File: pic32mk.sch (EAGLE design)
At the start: 31 parts, among them IC1 PIC32MK1024MCF100-I_PT, IC2 ADM3095EBRZ, IC3 PIC32MK1024MCF100-I_PT, IC4 MAX203ECWP

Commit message: up
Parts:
- added SV1: ICSP1, con-lstb:MA06-1
- added SV2: ICSP2, con-lstb:MA06-1
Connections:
- new net N$11: IC3.PGED1/OA1IN-/AN5/CTCMP/C1IN1-/RTCC/RPB3/RB3, SV1.4
- new net N$12: IC3.PGEC1/OA1IN+/AN4/C1IN1+/C1IN3-/C2IN3-/RPB2/RB2, SV1.5
- new net N$13: IC1.PGED1/OA1IN-/AN5/CTCMP/C1IN1-/RTCC/RPB3/RB3, SV2.4
- new net N$14: IC1.PGEC1/OA1IN+/AN4/C1IN1+/C1IN3-/C2IN3-/RPB2/RB2, SV2.5
- net +3V3: now also SV1.3, SV2.3
- net N$2: now also SV2.1
- net N$5: now also SV1.1
- net VSS: now also SV1.2, SV2.2
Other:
- moved on the sheet: U$1
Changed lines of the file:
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@@
 <class number="0" name="default" width="0" drill="0">
 </class>
-<class number="1" name="icurrent" width="0.0127" drill="0">
+<class number="1" name="icurrent" width="0.2159" drill="0">
 </class>
 </classes>
@@
 <part name="VSS25" library="supply1" library_urn="urn:adsk.eagle:library:371" deviceset="VSS" device=""/>
 <part name="VSS26" library="supply1" library_urn="urn:adsk.eagle:library:371" deviceset="VSS" device=""/>
+<part name="SV1" library="con-lstb" library_urn="urn:adsk.eagle:library:162" deviceset="MA06-1" device="" package3d_urn="urn:adsk.eagle:package:8340/1" value="ICSP1"/>
+<part name="VSS27" library="supply1" library_urn="urn:adsk.eagle:library:371" deviceset="VSS" device=""/>
+<part name="+3V2" library="supply1" library_urn="urn:adsk.eagle:library:371" deviceset="+3V3" device=""/>
+<part name="SV2" library="con-lstb" library_urn="urn:adsk.eagle:library:162" deviceset="MA06-1" device="" package3d_urn="urn:adsk.eagle:package:8340/1" value="ICSP2"/>
+<part name="VSS28" library="supply1" library_urn="urn:adsk.eagle:library:371" deviceset="VSS" device=""/>
+<part name="+3V3" library="supply1" library_urn="urn:adsk.eagle:library:371" deviceset="+3V3" device=""/>
 </parts>
 <sheets>
@@
 <attribute name="VALUE" x="208.28" y="-127" size="1.778" layer="96"/>
 </instance>
-<instance part="U$1" gate="G$1" x="-43.18" y="-101.6" smashed="yes">
-<attribute name="VALUE" x="-50.81086875" y="-88.8819" size="2.54361875" layer="96"/>
-<attribute name="NAME" x="-61.009" y="-65.942" size="1.7829" layer="95"/>
+<instance part="U$1" gate="G$1" x="-66.04" y="-99.06" smashed="yes">
+<attribute name="VALUE" x="-73.67086875" y="-86.3419" size="2.54361875" layer="96"/>
+<attribute name="NAME" x="-83.869" y="-63.402" size="1.7829" layer="95"/>
 </instance>
 <instance part="U$2" gate="G$1" x="-124.46" y="416.56" smashed="yes">
@@
 <attribute name="VALUE" x="-121.285" y="342.265" size="1.778" layer="96"/>
 </instance>
-<instance part="SUPPLY2" gate="GND" x="-43.18" y="-139.7" smashed="yes">
-<attribute name="VALUE" x="-45.085" y="-142.875" size="1.778" layer="96"/>
-</instance>
-<instance part="P+4" gate="VCC" x="-43.18" y="-63.5" smashed="yes">
-<attribute name="VALUE" x="-45.72" y="-66.04" size="1.778" layer="96" rot="R90"/>
+<instance part="SUPPLY2" gate="GND" x="-66.04" y="-137.16" smashed="yes">
+<attribute name="VALUE" x="-67.945" y="-140.335" size="1.778" layer="96"/>
+</instance>
+<instance part="P+4" gate="VCC" x="-66.04" y="-58.42" smashed="yes">
+<attribute name="VALUE" x="-68.58" y="-60.96" size="1.778" layer="96" rot="R90"/>
 </instance>
 <instance part="C10" gate="G$1" x="-96.52" y="365.76" smashed="yes">
@@
 <instance part="VSS26" gate="G$1" x="-86.36" y="358.14" smashed="yes">
 <attribute name="VALUE" x="-88.9" y="353.06" size="1.778" layer="96" rot="R90"/>
+</instance>
+<instance part="SV1" gate="1" x="-63.5" y="200.66" smashed="yes">
+<attribute name="VALUE" x="-64.77" y="187.96" size="1.778" layer="96"/>
+<attribute name="NAME" x="-64.77" y="209.042" size="1.778" layer="95"/>
+</instance>
+<instance part="VSS27" gate="G$1" x="-48.26" y="185.42" smashed="yes">
+<attribute name="VALUE" x="-50.8" y="180.34" size="1.778" layer="96" rot="R90"/>
+</instance>
+<instance part="+3V2" gate="G$1" x="-48.26" y="213.36" smashed="yes">
+<attribute name="VALUE" x="-50.8" y="208.28" size="1.778" layer="96" rot="R90"/>
+</instance>
+<instance part="SV2" gate="1" x="-30.48" y="-96.52" smashed="yes">
+<attribute name="VALUE" x="-31.75" y="-109.22" size="1.778" layer="96"/>
+<attribute name="NAME" x="-31.75" y="-88.138" size="1.778" layer="95"/>
+</instance>
+<instance part="VSS28" gate="G$1" x="-15.24" y="-111.76" smashed="yes">
+<attribute name="VALUE" x="-17.78" y="-116.84" size="1.778" layer="96" rot="R90"/>
+</instance>
+<instance part="+3V3" gate="G$1" x="-15.24" y="-83.82" smashed="yes">
+<attribute name="VALUE" x="-17.78" y="-88.9" size="1.778" layer="96" rot="R90"/>
 </instance>
 </instances>
@@
 <pinref part="IC1" gate="G$1" pin="!MCLR"/>
 <pinref part="R1" gate="G$1" pin="2"/>
-<wire x1="12.7" y1="15.24" x2="-25.4" y2="15.24" width="0.1524" layer="91"/>
+<wire x1="12.7" y1="15.24" x2="-22.86" y2="15.24" width="0.1524" layer="91"/>
 <junction x="-25.4" y="15.24"/>
 <junction x="12.7" y="15.24"/>
-</segment>
-</net>
-<net name="VDD" class="0">
+<wire x1="-22.86" y1="15.24" x2="-25.4" y2="15.24" width="0.1524" layer="91"/>
+<wire x1="-25.4" y1="15.24" x2="-22.86" y2="15.24" width="0.1524" layer="91"/>
+<wire x1="-22.86" y1="15.24" x2="-22.86" y2="-71.12" width="0.1524" layer="91"/>
+<pinref part="SV2" gate="1" pin="1"/>
+<wire x1="-22.86" y1="-104.14" x2="2.54" y2="-104.14" width="0.1524" layer="91"/>
+<wire x1="2.54" y1="-104.14" x2="2.54" y2="-71.12" width="0.1524" layer="91"/>
+<junction x="2.54" y="-104.14"/>
+<junction x="-22.86" y="-104.14"/>
+<wire x1="-22.86" y1="-71.12" x2="2.54" y2="-71.12" width="0.1524" layer="91"/>
+<junction x="-22.86" y="15.24"/>
+</segment>
+</net>
+<net name="VDD" class="1">
 <segment>
 <pinref part="R2" gate="G$1" pin="2"/>
@@
 </segment>
 </net>
-<net name="VSS" class="0">
+<net name="VSS" class="1">
 <segment>
 <pinref part="C1" gate="G$1" pin="2"/>
@@
 <junction x="-86.36" y="360.68"/>
 </segment>
+<segment>
+<pinref part="SV1" gate="1" pin="2"/>
+<wire x1="-55.88" y1="195.58" x2="-48.26" y2="195.58" width="0.1524" layer="91"/>
+<wire x1="-48.26" y1="195.58" x2="-48.26" y2="187.96" width="0.1524" layer="91"/>
+<pinref part="VSS27" gate="G$1" pin="VSS"/>
+<junction x="-48.26" y="187.96"/>
+<junction x="-55.88" y="195.58"/>
+</segment>
+<segment>
+<pinref part="SV2" gate="1" pin="2"/>
+<wire x1="-22.86" y1="-101.6" x2="-15.24" y2="-101.6" width="0.1524" layer="91"/>
+<wire x1="-15.24" y1="-101.6" x2="-15.24" y2="-109.22" width="0.1524" layer="91"/>
+<pinref part="VSS28" gate="G$1" pin="VSS"/>
+<junction x="-15.24" y="-109.22"/>
+<junction x="-22.86" y="-101.6"/>
+</segment>
 </net>
 <net name="+5V" class="1">
@@
 <pinref part="IC3" gate="G$1" pin="!MCLR"/>
 <pinref part="R3" gate="G$1" pin="2"/>
-<wire x1="10.16" y1="312.42" x2="-33.02" y2="312.42" width="0.1524" layer="91"/>
+<wire x1="10.16" y1="312.42" x2="-27.94" y2="312.42" width="0.1524" layer="91"/>
+<junction x="10.16" y="312.42"/>
+<pinref part="SV1" gate="1" pin="1"/>
+<wire x1="-30.48" y1="312.42" x2="-33.02" y2="312.42" width="0.1524" layer="91"/>
+<wire x1="-55.88" y1="193.04" x2="-30.48" y2="193.04" width="0.1524" layer="91"/>
+<wire x1="-30.48" y1="193.04" x2="-30.48" y2="226.06" width="0.1524" layer="91"/>
+<wire x1="-30.48" y1="226.06" x2="-30.48" y2="312.42" width="0.1524" layer="91"/>
+<wire x1="-30.48" y1="312.42" x2="-27.94" y2="312.42" width="0.1524" layer="91"/>
 <junction x="-33.02" y="312.42"/>
-<junction x="10.16" y="312.42"/>
+<junction x="-30.48" y="312.42"/>
+<junction x="-30.48" y="193.04"/>
+<junction x="-55.88" y="193.04"/>
+<junction x="-30.48" y="226.06"/>
 </segment>
 </net>
@@
 <pinref part="U$1" gate="G$1" pin="VCC"/>
 <pinref part="P+4" gate="VCC" pin="VCC"/>
+<wire x1="-66.04" y1="-63.5" x2="-66.04" y2="-60.96" width="0.1524" layer="91"/>
 </segment>
 </net>
@@
 <pinref part="+3V1" gate="G$1" pin="+3V3"/>
 <junction x="-129.54" y="368.3"/>
+</segment>
+<segment>
+<pinref part="SV1" gate="1" pin="3"/>
+<wire x1="-55.88" y1="198.12" x2="-48.26" y2="198.12" width="0.1524" layer="91"/>
+<wire x1="-48.26" y1="198.12" x2="-48.26" y2="210.82" width="0.1524" layer="91"/>
+<junction x="-55.88" y="198.12"/>
+<pinref part="+3V2" gate="G$1" pin="+3V3"/>
+<junction x="-48.26" y="210.82"/>
+</segment>
+<segment>
+<pinref part="SV2" gate="1" pin="3"/>
+<wire x1="-22.86" y1="-99.06" x2="-15.24" y2="-99.06" width="0.1524" layer="91"/>
+<wire x1="-15.24" y1="-99.06" x2="-15.24" y2="-86.36" width="0.1524" layer="91"/>
+<junction x="-22.86" y="-99.06"/>
+<pinref part="+3V3" gate="G$1" pin="+3V3"/>
+<junction x="-15.24" y="-86.36"/>
 </segment>
 </net>
@@
 </segment>
 </net>
+<net name="N$11" class="0">
+<segment>
+<pinref part="SV1" gate="1" pin="4"/>
+<wire x1="-55.88" y1="200.66" x2="-10.16" y2="200.66" width="0.1524" layer="91"/>
+<pinref part="IC3" gate="G$1" pin="PGED1/OA1IN-/AN5/CTCMP/C1IN1-/RTCC/RPB3/RB3"/>
+<wire x1="-10.16" y1="200.66" x2="55.88" y2="200.66" width="0.1524" layer="91"/>
+<wire x1="55.88" y1="200.66" x2="55.88" y2="208.28" width="0.1524" layer="91"/>
+<junction x="-55.88" y="200.66"/>
+<junction x="55.88" y="208.28"/>
+<junction x="-10.16" y="200.66"/>
+</segment>
+</net>
+<net name="N$12" class="0">
+<segment>
+<pinref part="SV1" gate="1" pin="5"/>
+<wire x1="-55.88" y1="203.2" x2="-10.16" y2="203.2" width="0.1524" layer="91"/>
+<pinref part="IC3" gate="G$1" pin="PGEC1/OA1IN+/AN4/C1IN1+/C1IN3-/C2IN3-/RPB2/RB2"/>
+<wire x1="-10.16" y1="203.2" x2="53.34" y2="203.2" width="0.1524" layer="91"/>
+<wire x1="53.34" y1="203.2" x2="53.34" y2="208.28" width="0.1524" layer="91"/>
+<junction x="-55.88" y="203.2"/>
+<junction x="53.34" y="208.28"/>
+<junction x="-10.16" y="203.2"/>
+</segment>
+</net>
+<net name="N$13" class="0">
+<segment>
+<pinref part="SV2" gate="1" pin="4"/>
+<wire x1="-22.86" y1="-96.52" x2="58.42" y2="-96.52" width="0.1524" layer="91"/>
+<junction x="-22.86" y="-96.52"/>
+<pinref part="IC1" gate="G$1" pin="PGED1/OA1IN-/AN5/CTCMP/C1IN1-/RTCC/RPB3/RB3"/>
+<wire x1="58.42" y1="-88.9" x2="58.42" y2="-96.52" width="0.1524" layer="91"/>
+<junction x="58.42" y="-88.9"/>
+</segment>
+</net>
+<net name="N$14" class="0">
+<segment>
+<pinref part="SV2" gate="1" pin="5"/>
+<wire x1="-22.86" y1="-93.98" x2="55.88" y2="-93.98" width="0.1524" layer="91"/>
+<junction x="-22.86" y="-93.98"/>
+<pinref part="IC1" gate="G$1" pin="PGEC1/OA1IN+/AN4/C1IN1+/C1IN3-/C2IN3-/RPB2/RB2"/>
+<wire x1="55.88" y1="-88.9" x2="55.88" y2="-93.98" width="0.1524" layer="91"/>
+<junction x="55.88" y="-88.9"/>
+</segment>
+</net>

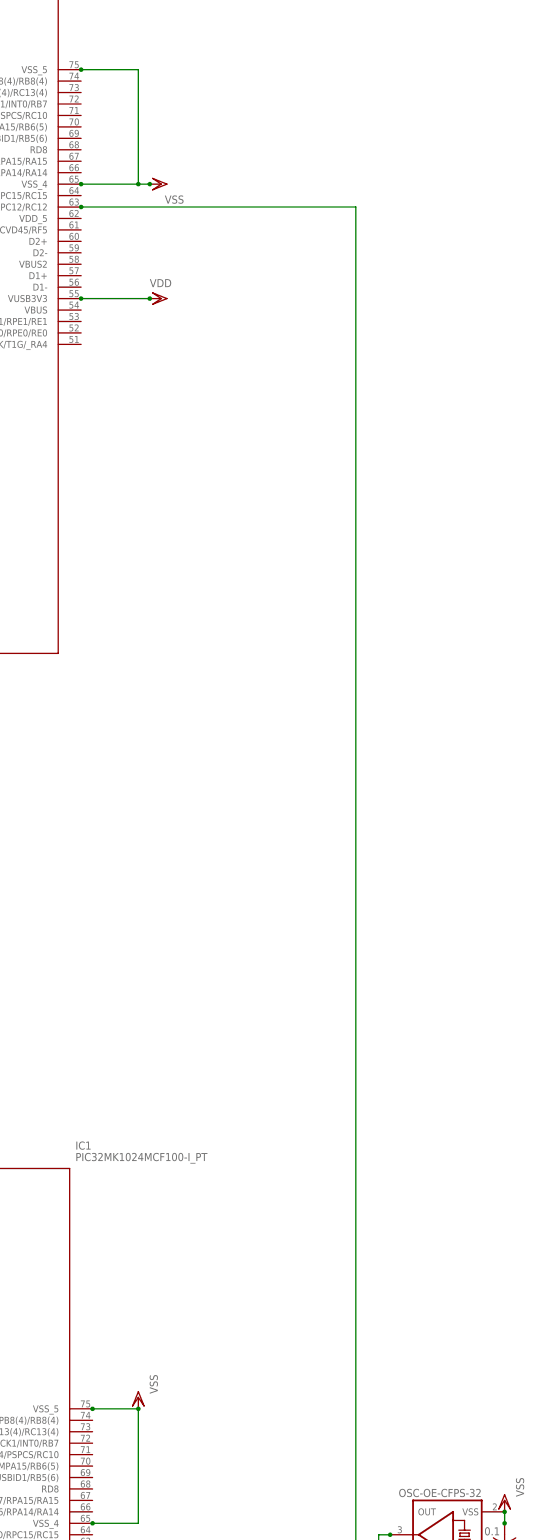
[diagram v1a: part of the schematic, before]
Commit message: up
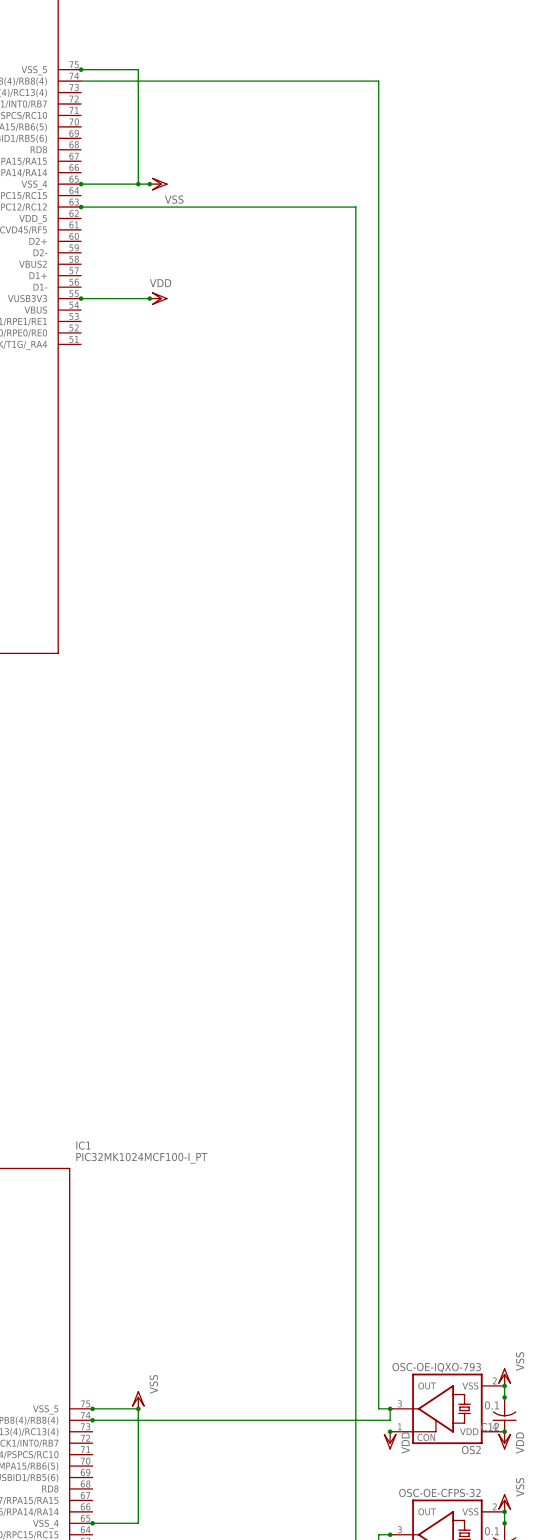
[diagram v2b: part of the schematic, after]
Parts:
- added C12: 0.1, rcl:C-USC0805
- added OS2: OSC-OE-IQXO-793, IQD-Frequency-Products:OSC-OE-IQXO-793
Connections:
- new net N$16: IC1.SOSCO/RPB8(4)/RB8(4), IC3.SOSCO/RPB8(4)/RB8(4), OS2.OUT
- net VDD: now also C12.1, OS2.CON, OS2.VDD
- net VSS: now also C12.2, OS2.VSS
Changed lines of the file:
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@@
 <part name="VSS28" library="supply1" library_urn="urn:adsk.eagle:library:371" deviceset="VSS" device=""/>
 <part name="+3V3" library="supply1" library_urn="urn:adsk.eagle:library:371" deviceset="+3V3" device=""/>
+<part name="OS2" library="IQD-Frequency-Products" library_urn="urn:adsk.eagle:library:90" deviceset="OSC-OE" device="-IQXO-793" package3d_urn="urn:adsk.eagle:package:3371/1"/>
+<part name="C12" library="rcl" library_urn="urn:adsk.eagle:library:334" deviceset="C-US" device="C0805" package3d_urn="urn:adsk.eagle:package:23617/2" value="0.1"/>
+<part name="VDD17" library="supply1" library_urn="urn:adsk.eagle:library:371" deviceset="VDD" device=""/>
+<part name="VDD18" library="supply1" library_urn="urn:adsk.eagle:library:371" deviceset="VDD" device=""/>
+<part name="VSS29" library="supply1" library_urn="urn:adsk.eagle:library:371" deviceset="VSS" device=""/>
 </parts>
 <sheets>
@@
 <instance part="+3V3" gate="G$1" x="-15.24" y="-83.82" smashed="yes">
 <attribute name="VALUE" x="-17.78" y="-88.9" size="1.778" layer="96" rot="R90"/>
+</instance>
+<instance part="OS2" gate="A" x="238.76" y="45.72" smashed="yes" rot="R180">
+<attribute name="NAME" x="246.38" y="37.465" size="1.778" layer="95" rot="R180"/>
+<attribute name="VALUE" x="246.38" y="55.88" size="1.778" layer="96" rot="R180"/>
+</instance>
+<instance part="C12" gate="G$1" x="251.46" y="43.18" smashed="yes" rot="R180">
+<attribute name="NAME" x="250.444" y="42.545" size="1.778" layer="95" rot="R180"/>
+<attribute name="VALUE" x="250.444" y="47.371" size="1.778" layer="96" rot="R180"/>
+</instance>
+<instance part="VDD17" gate="G$1" x="251.46" y="38.1" smashed="yes" rot="R180">
+<attribute name="VALUE" x="254" y="40.64" size="1.778" layer="96" rot="R270"/>
+</instance>
+<instance part="VDD18" gate="G$1" x="226.06" y="38.1" smashed="yes" rot="R180">
+<attribute name="VALUE" x="228.6" y="40.64" size="1.778" layer="96" rot="R270"/>
+</instance>
+<instance part="VSS29" gate="G$1" x="251.46" y="53.34" smashed="yes" rot="R180">
+<attribute name="VALUE" x="254" y="58.42" size="1.778" layer="96" rot="R270"/>
 </instance>
 </instances>
@@
 <wire x1="-96.52" y1="368.3" x2="-109.22" y2="368.3" width="0.1524" layer="91"/>
 </segment>
+<segment>
+<pinref part="OS2" gate="A" pin="VDD"/>
+<pinref part="C12" gate="G$1" pin="1"/>
+<pinref part="VDD17" gate="G$1" pin="VDD"/>
+<junction x="251.46" y="40.64"/>
+<pinref part="VDD17" gate="G$1" pin="VDD"/>
+</segment>
+<segment>
+<pinref part="OS2" gate="A" pin="CON"/>
+<pinref part="VDD18" gate="G$1" pin="VDD"/>
+<junction x="226.06" y="40.64"/>
+</segment>
 </net>
 <net name="VSS" class="1">
@@
 <junction x="-15.24" y="-109.22"/>
 <junction x="-22.86" y="-101.6"/>
+</segment>
+<segment>
+<pinref part="OS2" gate="A" pin="VSS"/>
+<pinref part="VSS29" gate="G$1" pin="VSS"/>
+<pinref part="C12" gate="G$1" pin="2"/>
+<wire x1="251.46" y1="48.26" x2="251.46" y2="50.8" width="0.1524" layer="91"/>
+<junction x="251.46" y="48.26"/>
+<junction x="251.46" y="50.8"/>
 </segment>
 </net>
@@
 </segment>
 </net>
+<net name="N$16" class="0">
+<segment>
+<pinref part="IC3" gate="G$1" pin="SOSCO/RPB8(4)/RB8(4)"/>
+<wire x1="157.48" y1="340.36" x2="223.52" y2="340.36" width="0.1524" layer="91"/>
+<wire x1="223.52" y1="340.36" x2="223.52" y2="45.72" width="0.1524" layer="91"/>
+<pinref part="IC1" gate="G$1" pin="SOSCO/RPB8(4)/RB8(4)"/>
+<wire x1="160.02" y1="43.18" x2="226.06" y2="43.18" width="0.1524" layer="91"/>
+<pinref part="OS2" gate="A" pin="OUT"/>
+<wire x1="226.06" y1="43.18" x2="226.06" y2="45.72" width="0.1524" layer="91"/>
+<junction x="160.02" y="43.18"/>
+<junction x="226.06" y="45.72"/>
+<wire x1="223.52" y1="45.72" x2="226.06" y2="45.72" width="0.1524" layer="91"/>
+</segment>
+</net>
